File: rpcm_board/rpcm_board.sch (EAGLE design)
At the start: 56 parts, among them Q4 DMG1012T, U1 SFW15R-1STE1LF, U2 SFW15R-1STE1LF, U3 DMG1012T, U4 MICROSD_SD_MODEMOLEX, U5 PAM2306DYPAA

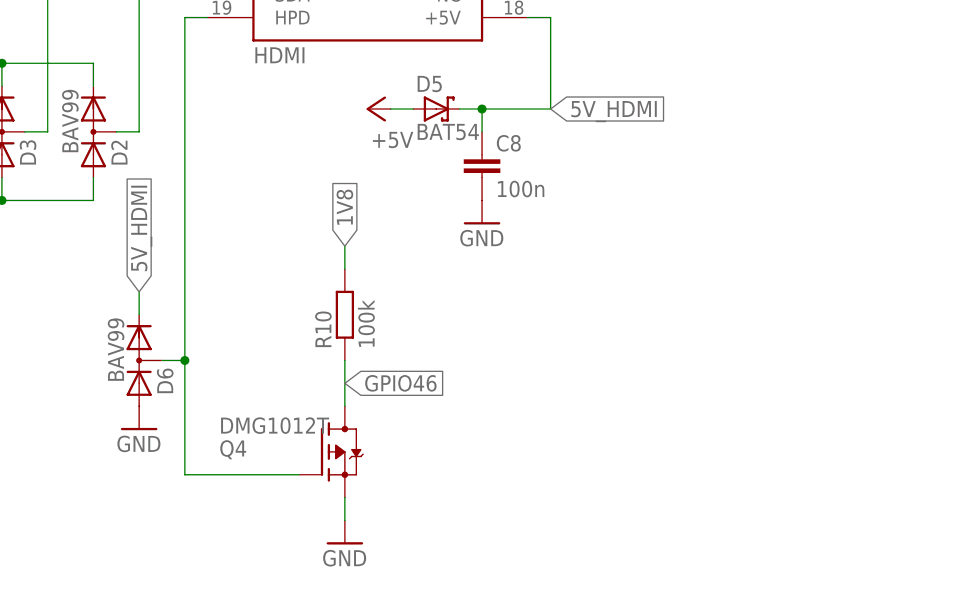
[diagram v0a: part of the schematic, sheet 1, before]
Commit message: before autorouter
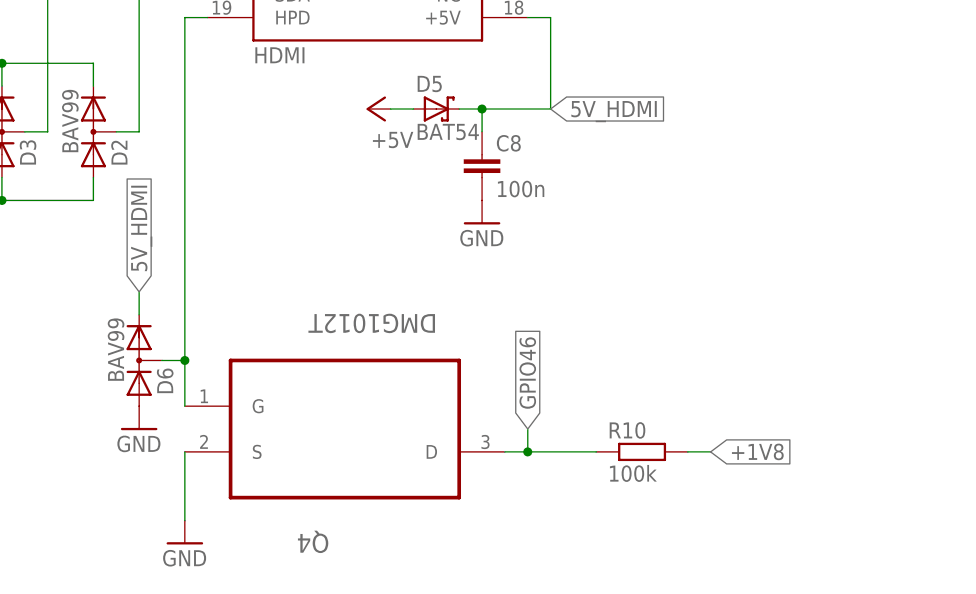
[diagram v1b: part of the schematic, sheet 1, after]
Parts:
- C8: device rcl:C-EUC0603 -> resistor:C-EUC0402
- Q4: device transistor-fet:BSA223SP -> openblw:DMG1012T
- R10, R18, R19: device rcl:R-EU_R0603 -> resistor:R-EU_R0402
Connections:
- removed net 1V8: R10.2
- net +1V8: now also R10.2
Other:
- moved on the sheet: R10
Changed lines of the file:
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@@
 <part name="D4" library="diode" deviceset="BAV199" device="" value="BAV99"/>
 <part name="D5" library="diode" deviceset="BAT54" device=""/>
-<part name="C8" library="rcl" deviceset="C-EU" device="C0603" value="100n"/>
+<part name="C8" library="resistor" deviceset="C-EU" device="C0402" value="100n"/>
 <part name="GND27" library="supply1" deviceset="GND" device=""/>
 <part name="P+9" library="supply1" deviceset="+5V" device=""/>
 <part name="GND12" library="supply1" deviceset="GND" device=""/>
 <part name="D6" library="diode" deviceset="BAV199" device="" value="BAV99"/>
-<part name="R10" library="rcl" deviceset="R-EU_" device="R0603" value="100k"/>
-<part name="Q4" library="transistor-fet" deviceset="BSA223SP" device="" value="DMG1012T"/>
+<part name="R10" library="resistor" deviceset="R-EU_" device="R0402" value="100k"/>
+<part name="Q4" library="openblw" deviceset="DMG1012T" device="" value="DMG1012T"/>
 <part name="GND14" library="supply1" deviceset="GND" device=""/>
 <part name="GND30" library="supply1" deviceset="GND" device=""/>
-<part name="R18" library="rcl" deviceset="R-EU_" device="R0603" value="1k8"/>
-<part name="R19" library="rcl" deviceset="R-EU_" device="R0603" value="1k8"/>
+<part name="R18" library="resistor" deviceset="R-EU_" device="R0402" value="1k8"/>
+<part name="R19" library="resistor" deviceset="R-EU_" device="R0402" value="1k8"/>
 <part name="P+10" library="supply1" deviceset="+5V" device=""/>
 <part name="P+11" library="supply1" deviceset="+5V" device=""/>
@@
 <instance part="GND12" gate="1" x="157.48" y="40.64"/>
 <instance part="D6" gate="G$1" x="182.88" y="27.94" rot="R270"/>
-<instance part="R10" gate="G$1" x="205.74" y="33.02" rot="R90"/>
-<instance part="Q4" gate="G$1" x="203.2" y="17.78" rot="MR180"/>
-<instance part="GND14" gate="1" x="205.74" y="7.62"/>
+<instance part="R10" gate="G$1" x="238.76" y="17.78"/>
+<instance part="Q4" gate="G$1" x="205.74" y="17.78" rot="MR180"/>
+<instance part="GND14" gate="1" x="187.96" y="7.62"/>
 <instance part="GND30" gate="1" x="182.88" y="20.32"/>
 <instance part="R18" gate="G$1" x="154.94" y="86.36" rot="R90"/>
@@
 <pinref part="Q4" gate="G$1" pin="S"/>
 <pinref part="GND14" gate="1" pin="GND"/>
-<wire x1="205.74" y1="10.16" x2="205.74" y2="12.7" width="0.1524" layer="91"/>
+<wire x1="187.96" y1="10.16" x2="187.96" y2="17.78" width="0.1524" layer="91"/>
 </segment>
 <segment>
@@
 <wire x1="353.06" y1="200.66" x2="355.6" y2="200.66" width="0.1524" layer="91"/>
 </segment>
+<segment>
+<pinref part="R10" gate="G$1" pin="2"/>
+<wire x1="243.84" y1="17.78" x2="246.38" y2="17.78" width="0.1524" layer="91"/>
+<label x="246.38" y="17.78" size="1.778" layer="95" xref="yes"/>
+</segment>
 </net>
 <net name="N$2" class="0">
@@
 <wire x1="66.04" y1="132.08" x2="66.04" y2="147.32" width="0.1524" layer="91"/>
 <label x="66.04" y="147.32" size="1.778" layer="95" rot="R90" xref="yes"/>
-</segment>
-</net>
-<net name="1V8" class="0">
-<segment>
-<pinref part="R10" gate="G$1" pin="2"/>
-<wire x1="205.74" y1="38.1" x2="205.74" y2="40.64" width="0.1524" layer="91"/>
-<label x="205.74" y="40.64" size="1.778" layer="95" rot="R90" xref="yes"/>
 </segment>
 </net>
@@
 <wire x1="190.5" y1="66.04" x2="187.96" y2="66.04" width="0.1524" layer="91"/>
 <pinref part="Q4" gate="G$1" pin="G"/>
-<wire x1="200.66" y1="15.24" x2="187.96" y2="15.24" width="0.1524" layer="91"/>
-<wire x1="187.96" y1="15.24" x2="187.96" y2="27.94" width="0.1524" layer="91"/>
+<wire x1="187.96" y1="22.86" x2="187.96" y2="27.94" width="0.1524" layer="91"/>
 <pinref part="D6" gate="G$1" pin="AC"/>
 <wire x1="187.96" y1="27.94" x2="185.42" y2="27.94" width="0.1524" layer="91"/>
@@
 <pinref part="R10" gate="G$1" pin="1"/>
 <pinref part="Q4" gate="G$1" pin="D"/>
-<wire x1="205.74" y1="27.94" x2="205.74" y2="22.86" width="0.1524" layer="91"/>
-<label x="205.74" y="25.4" size="1.778" layer="95" xref="yes"/>
-</segment>
-</net>
+<wire x1="233.68" y1="17.78" x2="226.06" y2="17.78" width="0.1524" layer="91"/>
+<label x="226.06" y="20.32" size="1.778" layer="95" rot="R90" xref="yes"/>
+<wire x1="226.06" y1="17.78" x2="223.52" y2="17.78" width="0.1524" layer="91"/>
+<wire x1="226.06" y1="17.78" x2="226.06" y2="20.32" width="0.1524" layer="91"/>
+<junction x="226.06" y="17.78"/>
+</segment>
+</net>
